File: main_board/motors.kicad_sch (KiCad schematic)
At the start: 18 parts

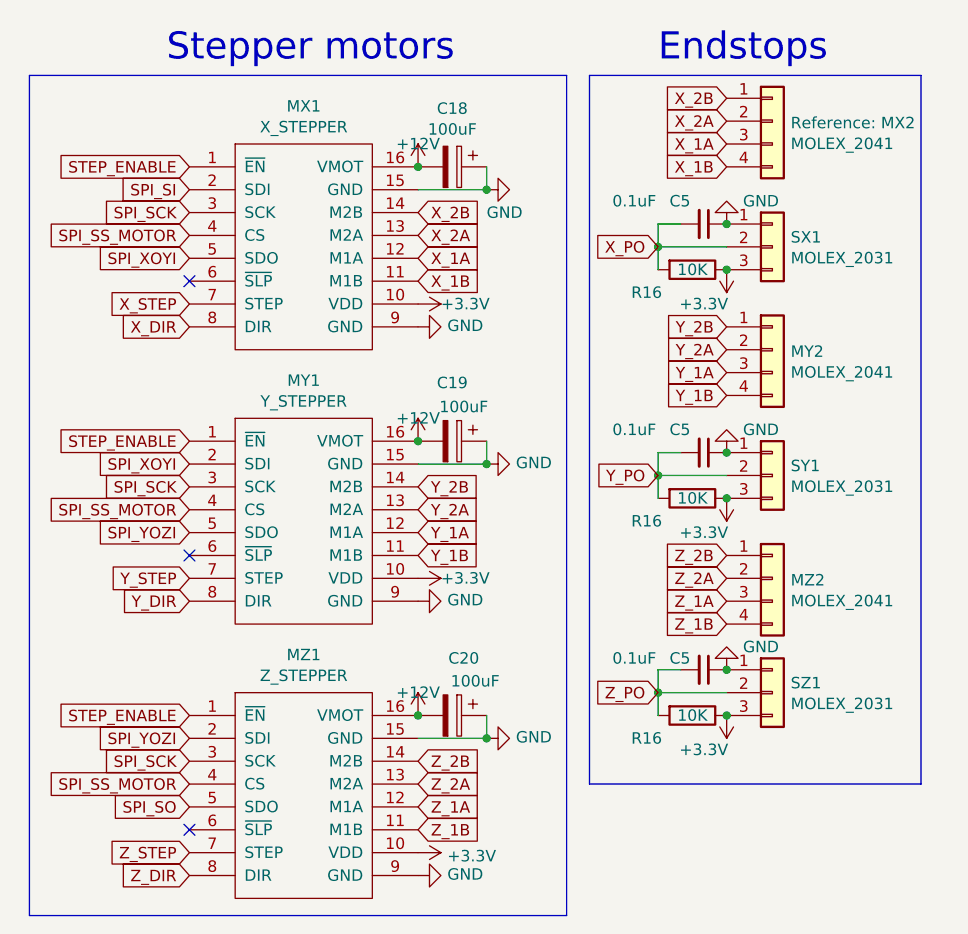
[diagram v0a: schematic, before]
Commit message: routed main board
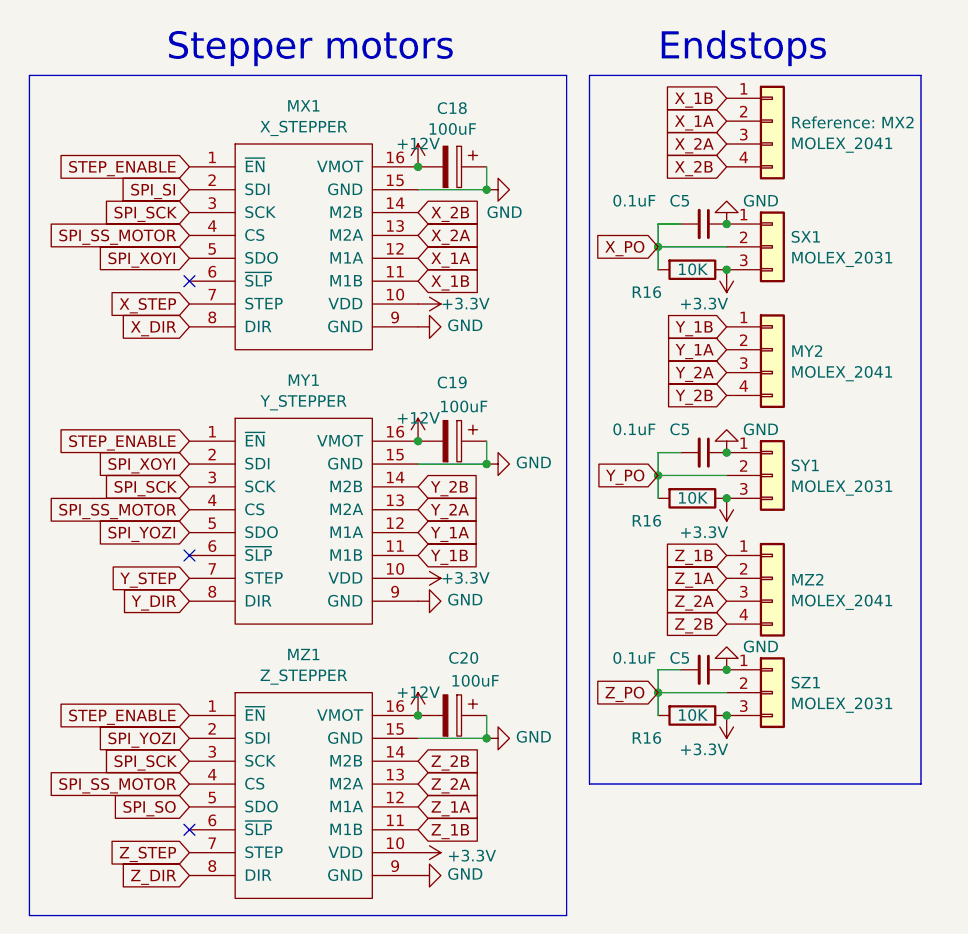
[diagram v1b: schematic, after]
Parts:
- C18, C19, C20: footprint Capacitor_THT:CP_Radial_D6.3mm_P2.50mm -> footprints:CP_Radial_D6.3mm_P2.50mm
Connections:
- net X_1A: now also MX2.2 (Pin_2); no longer MX2.3 (Pin_3)
- net X_1B: now also MX2.1 (Pin_1); no longer MX2.4 (Pin_4)
- net X_2A: now also MX2.3 (Pin_3); no longer MX2.2 (Pin_2)
- net X_2B: now also MX2.4 (Pin_4); no longer MX2.1 (Pin_1)
- net Y_1A: now also MY2.2 (Pin_2); no longer MY2.3 (Pin_3)
- net Y_1B: now also MY2.1 (Pin_1); no longer MY2.4 (Pin_4)
- net Y_2A: now also MY2.3 (Pin_3); no longer MY2.2 (Pin_2)
- net Y_2B: now also MY2.4 (Pin_4); no longer MY2.1 (Pin_1)
- net Z_1A: now also MZ2.2 (Pin_2); no longer MZ2.3 (Pin_3)
- net Z_1B: now also MZ2.1 (Pin_1); no longer MZ2.4 (Pin_4)
- net Z_2A: now also MZ2.3 (Pin_3); no longer MZ2.2 (Pin_2)
- net Z_2B: now also MZ2.4 (Pin_4); no longer MZ2.1 (Pin_1)
